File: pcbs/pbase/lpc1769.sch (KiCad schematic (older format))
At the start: 1 part

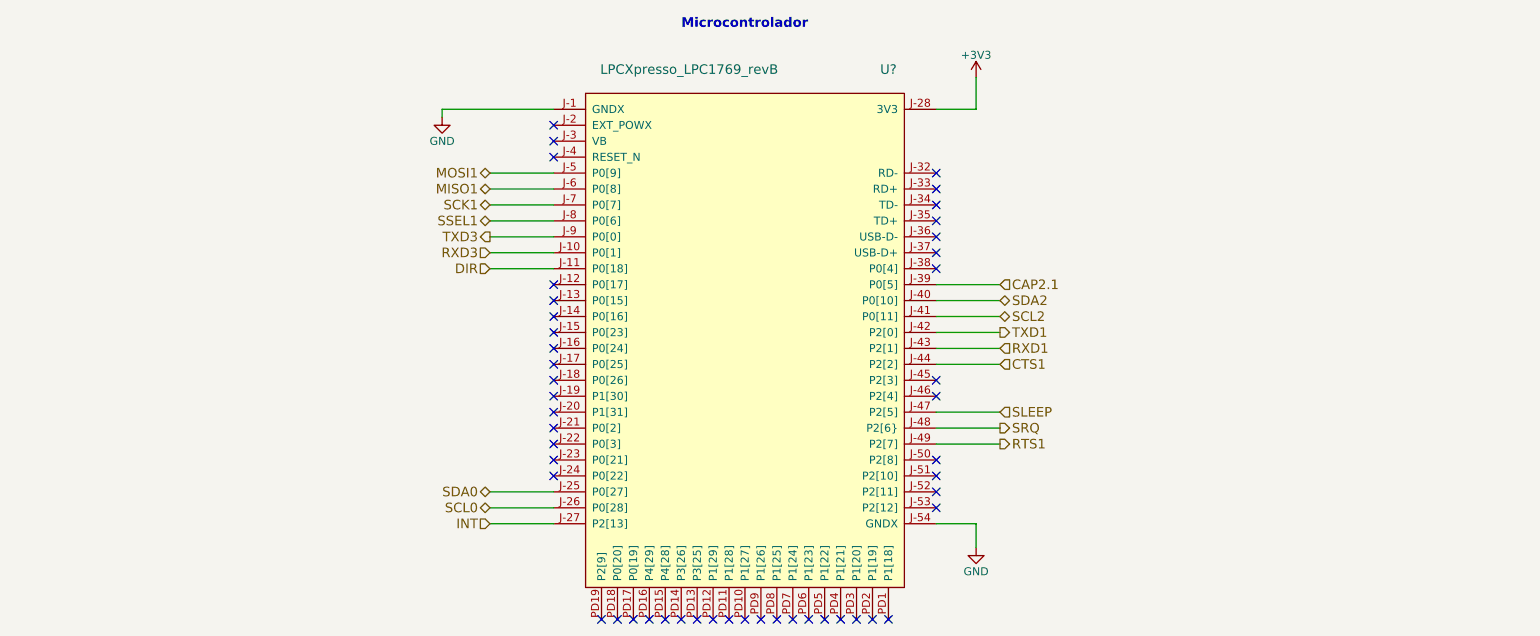
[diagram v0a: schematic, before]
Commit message: Test points
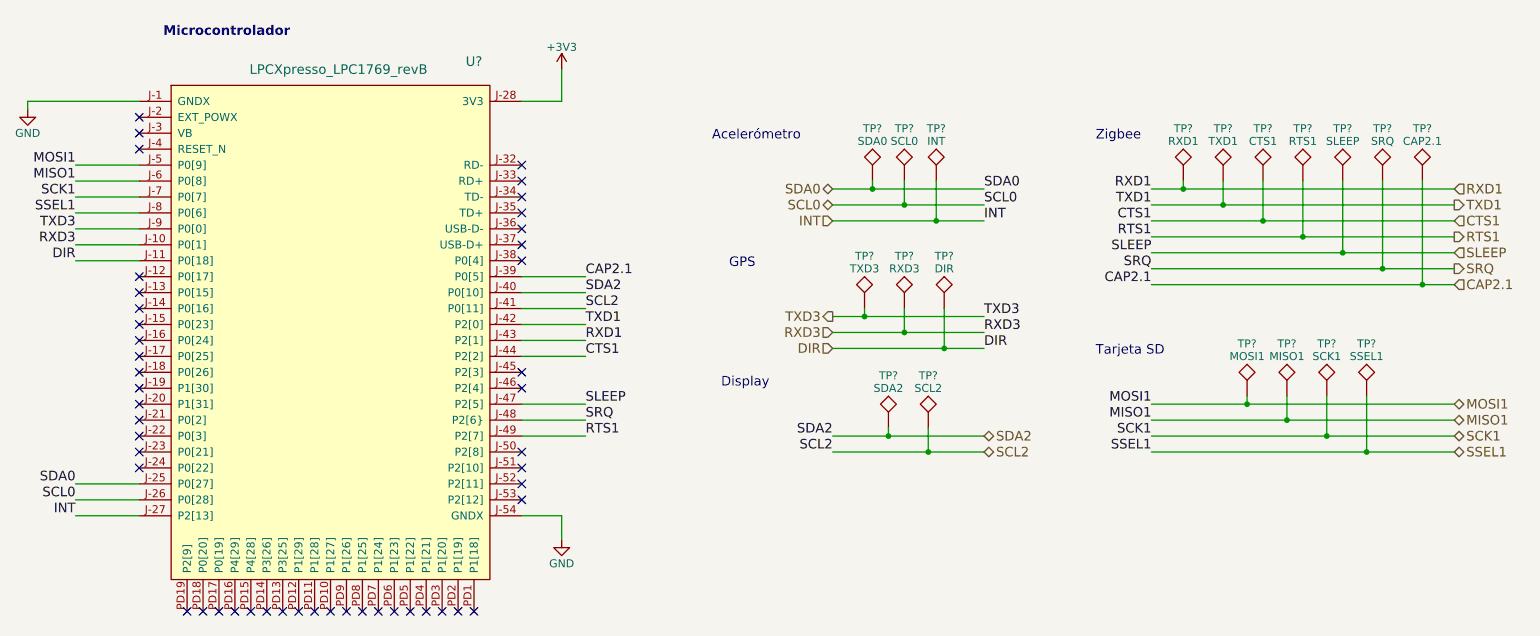
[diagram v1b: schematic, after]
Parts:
- added TP?: RXD1, symbol TEST
- added TP?: TXD1, symbol TEST
- added TP?: CTS1, symbol TEST
- added TP?: RTS1, symbol TEST
- added TP?: SLEEP, symbol TEST
- added TP?: SRQ, symbol TEST
- added TP?: CAP2.1, symbol TEST
- added TP?: INT, symbol TEST
- added TP?: SCL0, symbol TEST
- added TP?: SDA0, symbol TEST
- added TP?: SDA2, symbol TEST
- added TP?: SCL2, symbol TEST
- added TP?: MOSI1, symbol TEST
- added TP?: MISO1, symbol TEST
- added TP?: SCK1, symbol TEST
- added TP?: SSEL1, symbol TEST
- added TP?: TXD3, symbol TEST
- added TP?: RXD3, symbol TEST
- added TP?: DIR, symbol TEST
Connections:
- net CAP2.1: now also TP?.1
- net CTS1: now also TP?.1
- net DIR: now also TP?.1
- net INT: now also TP?.1
- net MISO1: now also TP?.1
- net MOSI1: now also TP?.1
- net RTS1: now also TP?.1
- net RXD1: now also TP?.1
- net RXD3: now also TP?.1
- net SCK1: now also TP?.1
- net SCL0: now also TP?.1
- net SCL2: now also TP?.1
- net SDA0: now also TP?.1
- net SDA2: now also TP?.1
- net SLEEP: now also TP?.1
- net SRQ: now also TP?.1
- net SSEL1: now also TP?.1
- net TXD1: now also TP?.1
- net TXD3: now also TP?.1
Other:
- note added: "Acelerómetro"
- note added: "Display"
- note added: "GPS\n"
- note added: "Tarjeta SD\n"
- note added: "Zigbee"
- moved on the sheet: U?
